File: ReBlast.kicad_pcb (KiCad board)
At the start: 2 copper layers, 50.7 x 64.9 mm, 23 parts, among them J1 MOS_8580_Socket, U1 74HC20, U2 74HC139, U3 ZN428E-8, U4 TLC272, U5 MOS_8580, U6 ADC0804

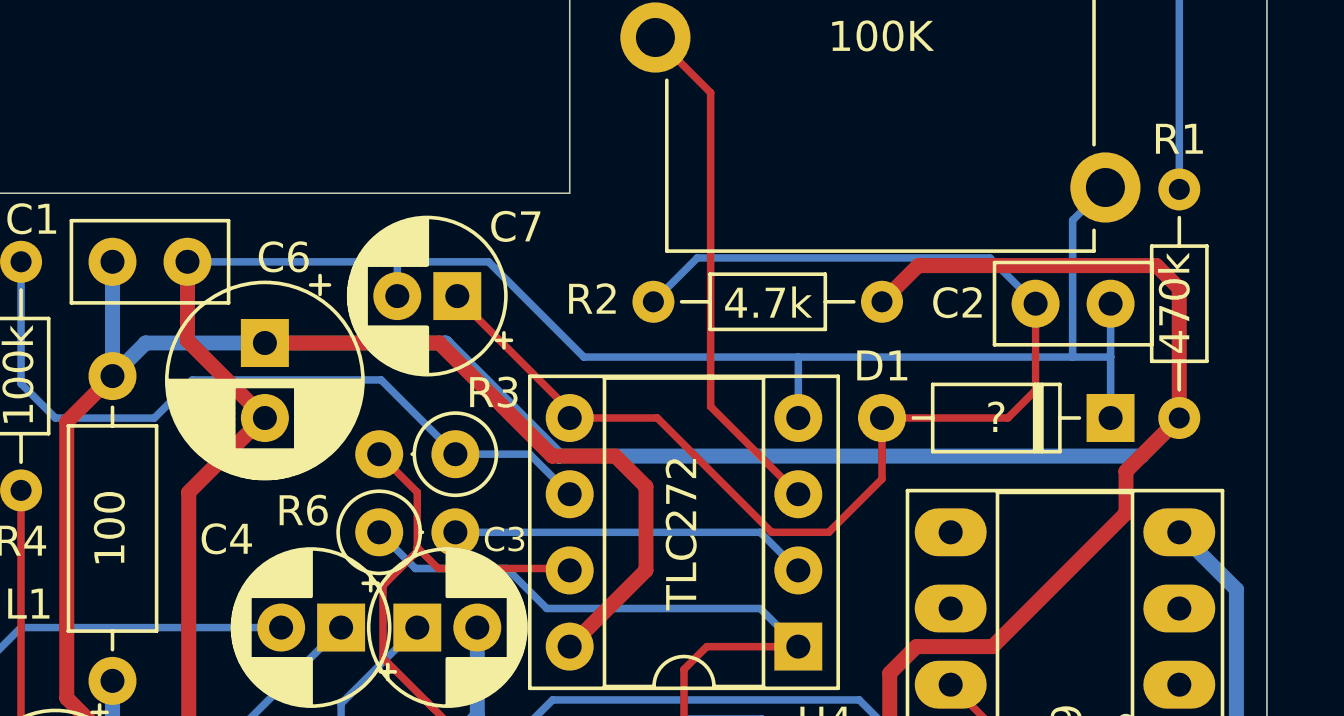
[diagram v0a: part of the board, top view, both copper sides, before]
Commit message: Fix DRC
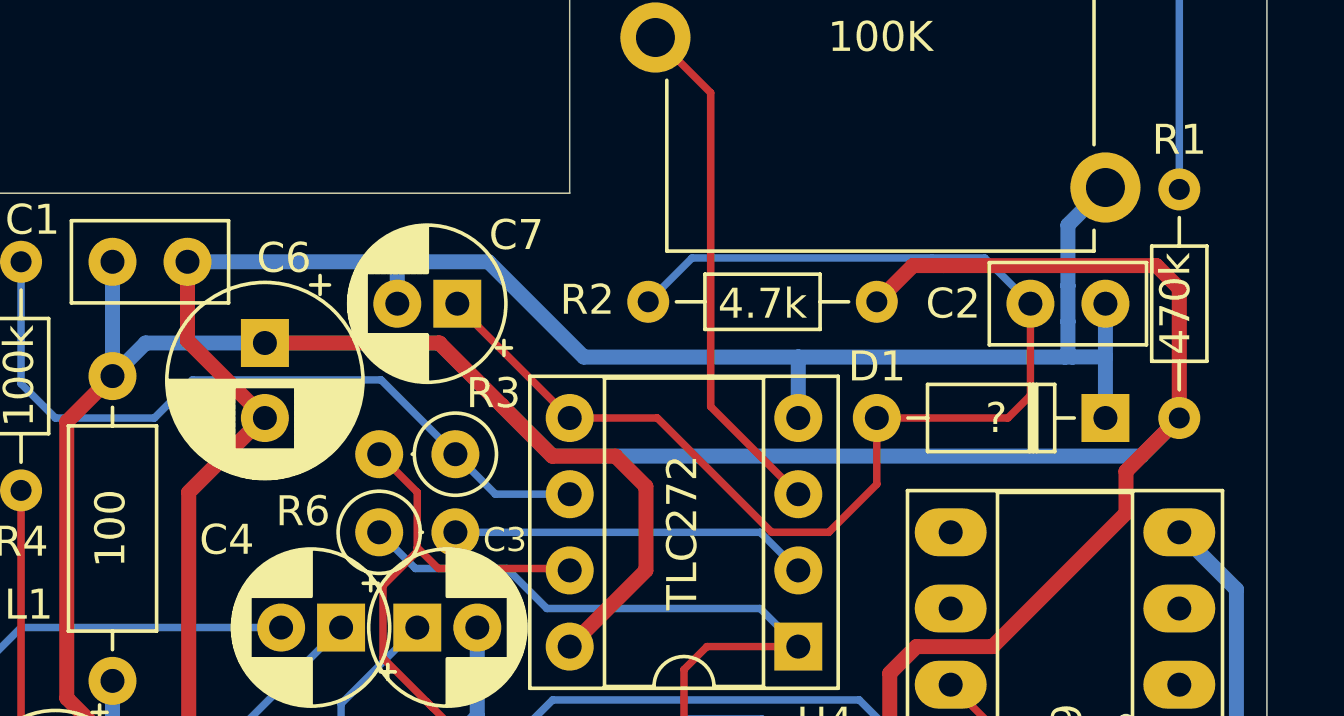
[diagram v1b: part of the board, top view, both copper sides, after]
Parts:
- moved C7 0.25 mm to (150.7, 80.5)
- moved R2 0.17 mm to (164.7, 80.5)
- moved C2 0.17 mm to (169.8, 80.5)
- moved D1 0.17 mm to (172.3, 84.3)
